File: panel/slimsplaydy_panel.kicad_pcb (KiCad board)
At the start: 2 copper layers, 155.6 x 195.5 mm, 179 parts

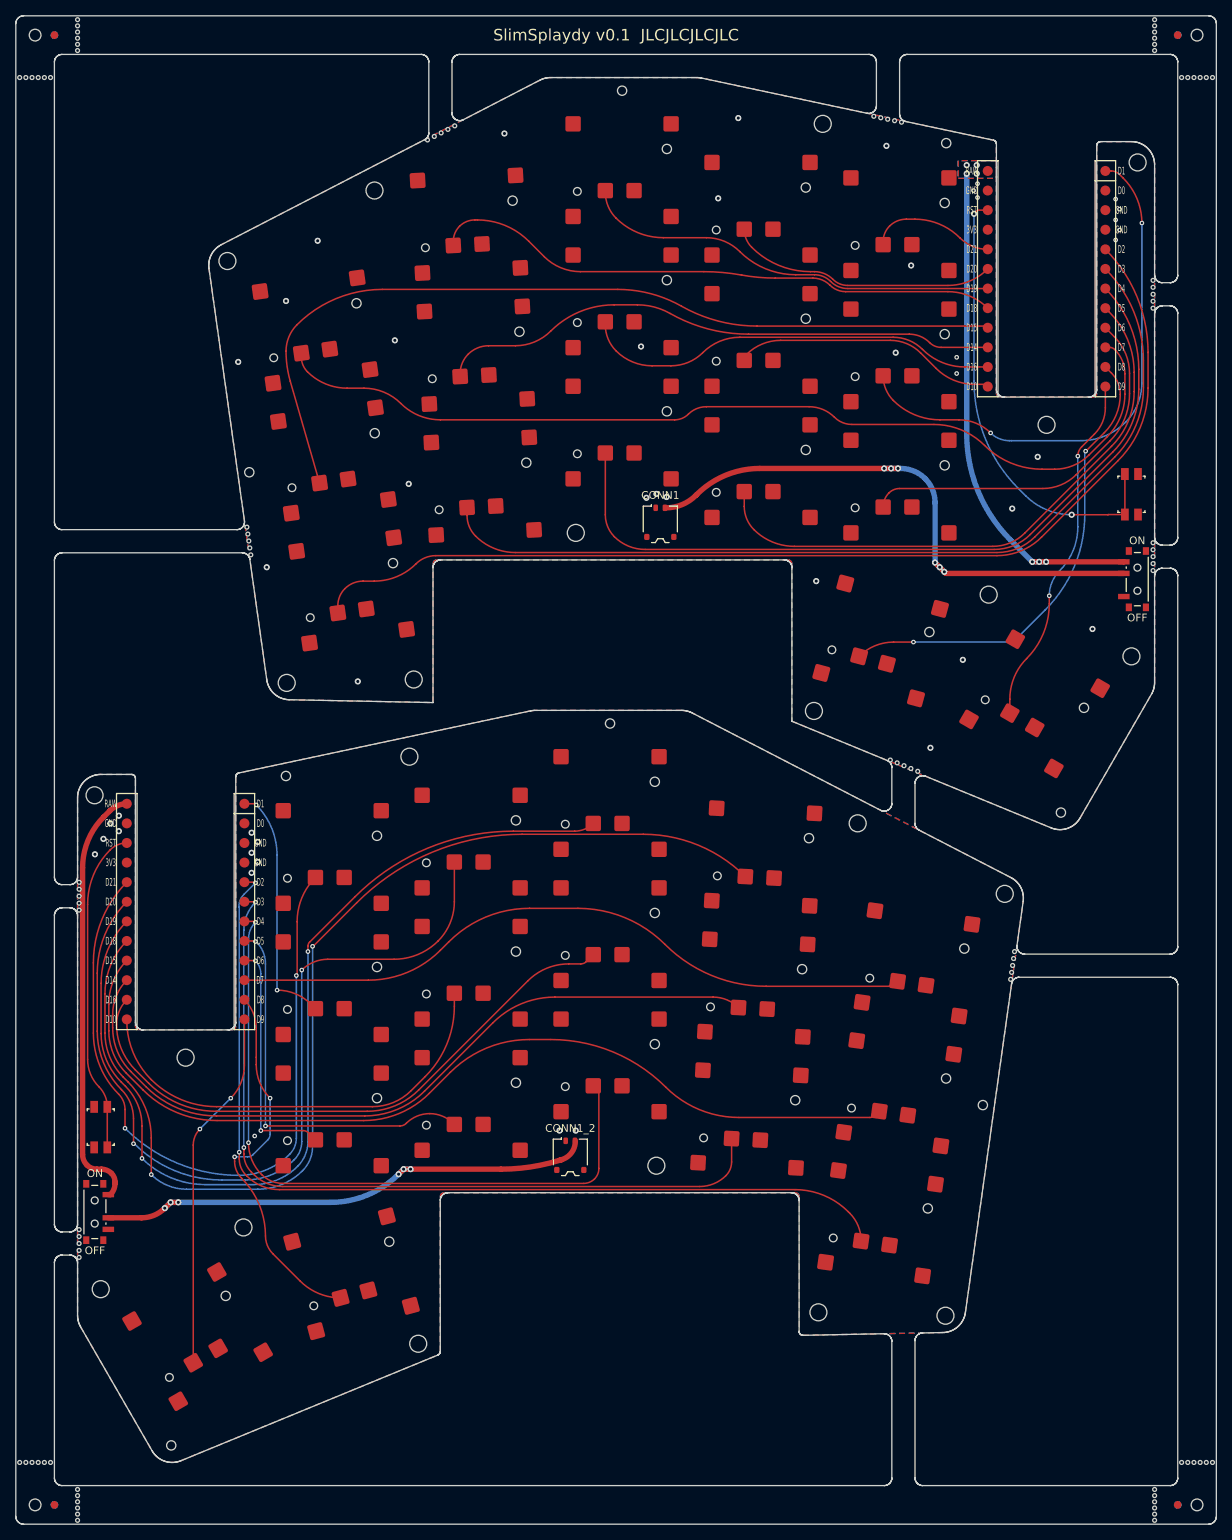
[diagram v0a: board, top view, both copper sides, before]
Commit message: Complete panel.
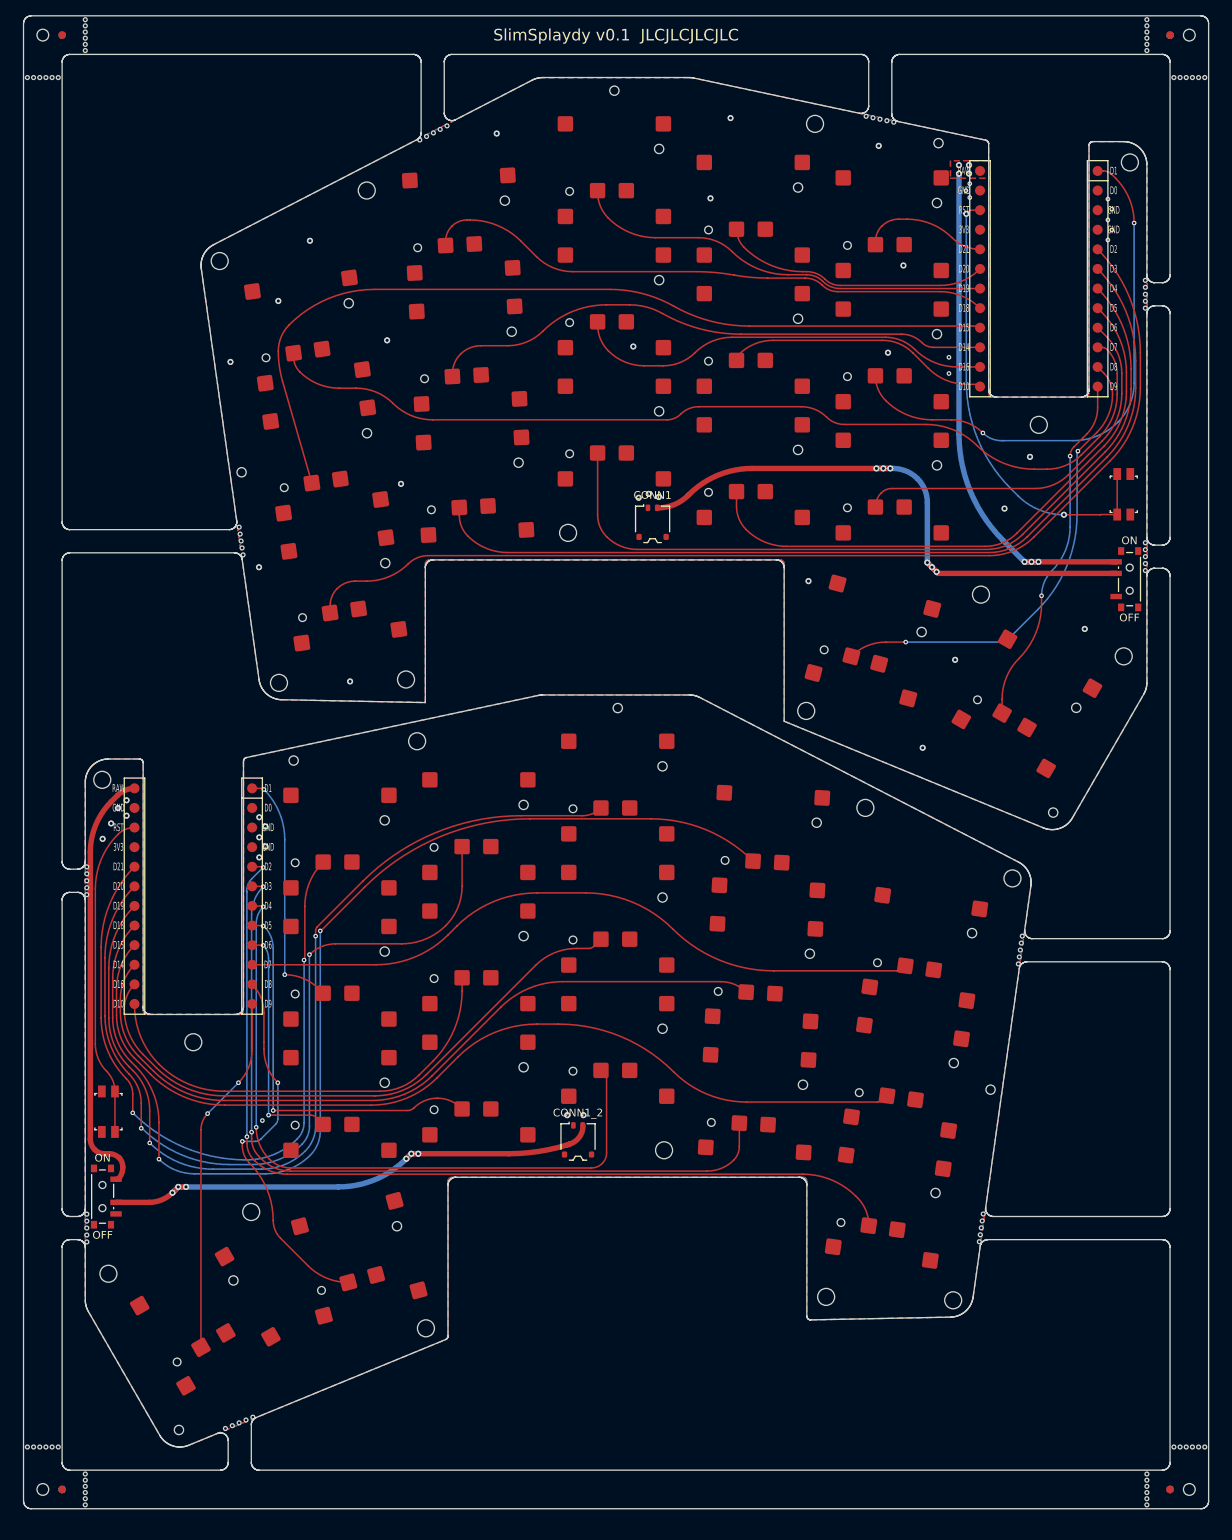
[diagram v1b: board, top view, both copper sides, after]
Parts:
- removed KiKit_MB_10_6, KiKit_MB_10_7: NPTH, NPTH
- added KiKit_MB_10_1: NPTH, NPTH, F.Cu at (196.1, 175.3)
- added KiKit_MB_18_2: NPTH, NPTH, F.Cu at (220.8, 205.5)
- added KiKit_MB_18_3: NPTH, NPTH, F.Cu at (221.6, 205.5)
- added KiKit_MB_18_4: NPTH, NPTH, F.Cu at (222.4, 205.5)
- added KiKit_MB_18_5: NPTH, NPTH, F.Cu at (223.2, 205.5)
- added KiKit_MB_18_6: NPTH, NPTH, F.Cu at (224.0, 205.5)
- added KiKit_MB_18_7: NPTH, NPTH, F.Cu at (224.8, 205.5)
- moved KiKit_MB_12_2 235.5 mm to (217.3, 20.5)
- moved KiKit_MB_12_3 235.5 mm to (217.3, 21.3)
- moved KiKit_MB_12_4 235.5 mm to (217.3, 22.1)
- moved KiKit_MB_12_5 235.5 mm to (217.3, 22.9)
- moved KiKit_MB_12_6 235.5 mm to (217.3, 23.7)
- moved KiKit_MB_12_7 235.5 mm to (217.3, 24.5)
- moved KiKit_MB_14_7 233.2 mm to (217.3, 213.0)
- moved KiKit_MB_14_6 233.1 mm to (217.3, 212.2)
- moved KiKit_MB_14_5 232.9 mm to (217.3, 211.4)
- moved KiKit_MB_14_4 232.8 mm to (217.3, 210.6)
- moved KiKit_MB_14_3 232.7 mm to (217.3, 209.8)
- moved KiKit_MB_14_2 232.5 mm to (217.3, 209.0)
- moved KiKit_MB_16_2 232.1 mm to (72.2, 205.5)
- moved KiKit_MB_16_3 232.1 mm to (73.0, 205.5)
- moved KiKit_MB_16_4 232.1 mm to (73.8, 205.5)
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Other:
- board size 155.6 x 195.5 mm -> 153.6 x 193.5 mm
